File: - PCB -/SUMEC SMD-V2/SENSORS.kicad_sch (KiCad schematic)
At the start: 20 parts, among them U4 QRE1113, U5 QRE1113, U6 QRE1113

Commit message: cleanup
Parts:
- U4, U5, U6: footprint sumec_library:OnSemi_CASE100AQ - QRE1113 -> (none)
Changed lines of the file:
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@@
       (effects (font (size 1.27 1.27)) (justify left))
     )
-    (property "Footprint" "sumec_library:OnSemi_CASE100AQ - QRE1113" (at 218.44 92.71 0)
+    (property "Footprint" "" (at 218.44 92.71 0)
       (effects (font (size 1.27 1.27)) hide)
     )
@@
       (effects (font (size 1.27 1.27)) (justify left))
     )
-    (property "Footprint" "sumec_library:OnSemi_CASE100AQ - QRE1113" (at 182.88 92.71 0)
+    (property "Footprint" "" (at 182.88 92.71 0)
       (effects (font (size 1.27 1.27)) hide)
     )
@@
       (effects (font (size 1.27 1.27)) (justify left))
     )
-    (property "Footprint" "sumec_library:OnSemi_CASE100AQ - QRE1113" (at 200.66 92.71 0)
-      (effects (font (size 1.27 1.27)) hide)
-    )
+    (property "Footprint" "" (at 200.66 92.71 0)
+      (effects (font (size 1.27 1.27)) hide)
+    )

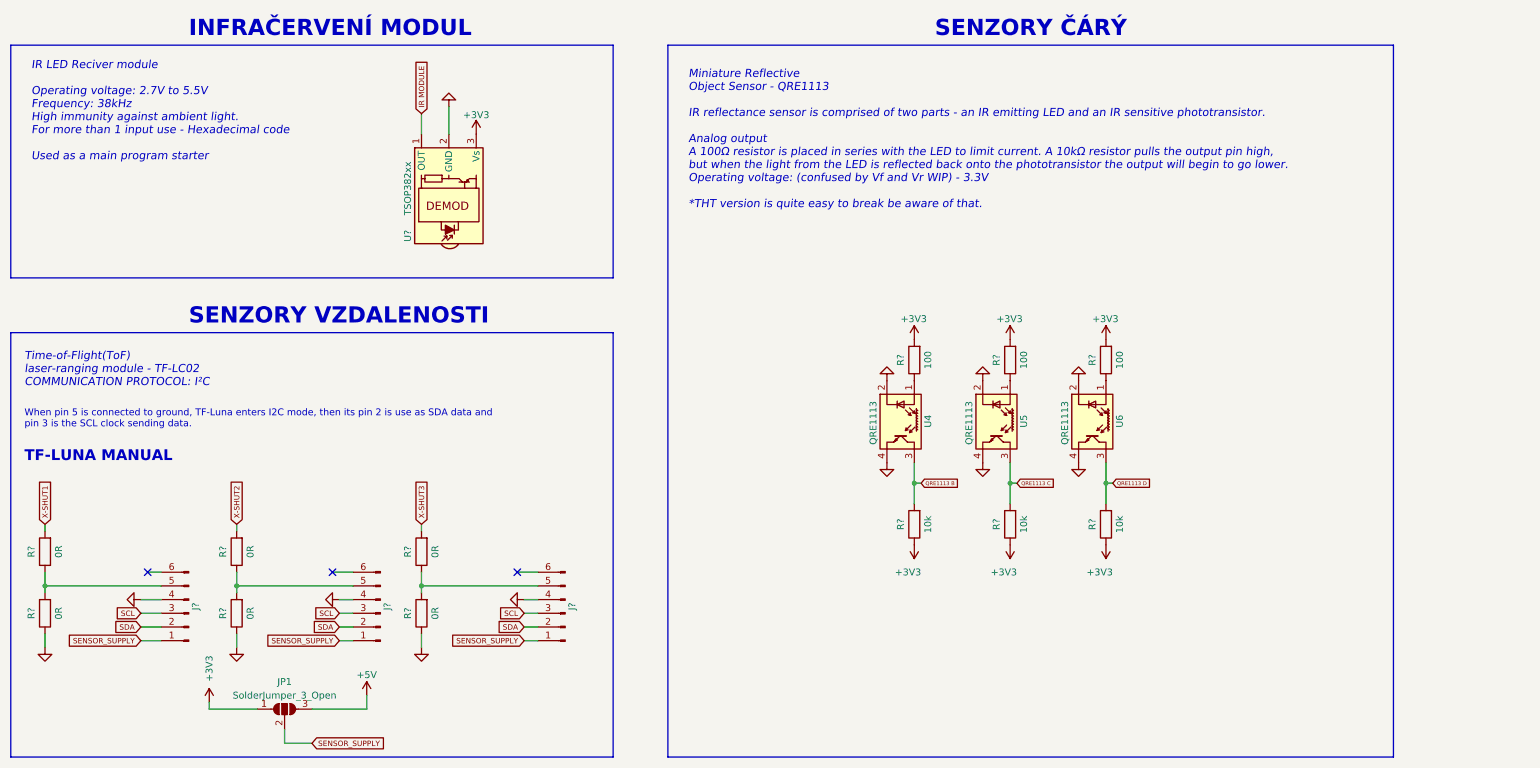
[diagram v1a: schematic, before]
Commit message: sumec SMD V2 schematic update
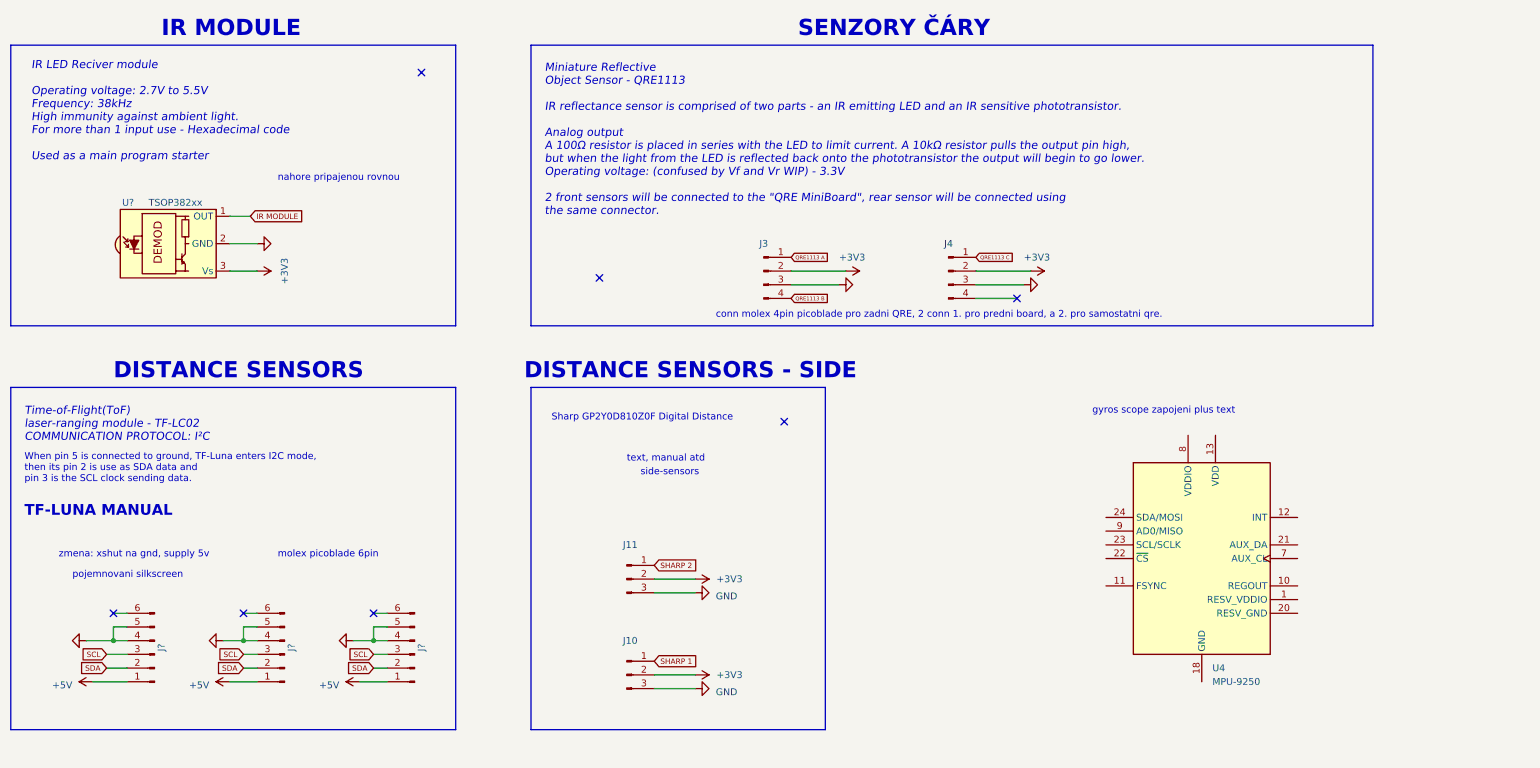
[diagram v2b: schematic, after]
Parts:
- removed J?: Conn_01x06_Pin, Connector_JST:JST_SH_BM06B-SRSS-TB_1x06-1MP_P1.00mm_Vertical, symbol Connector:Conn_01x06_Pin
- removed JP1: SolderJumper_3_Open, Jumper:SolderJumper-3_P2.0mm_Open_TrianglePad1.0x1.5mm, symbol Jumper:SolderJumper_3_Open
- removed R? (x3): 100, Resistor_SMD:R_1206_3216Metric, symbol Device:R
- removed R? (x6): 0R, Resistor_SMD:R_1206_3216Metric, symbol Device:R
- removed R? (x3): 10k, Resistor_SMD:R_1206_3216Metric, symbol Device:R
- removed U4, U5, U6: QRE1113, symbol Sensor_Proximity:QRE1113
- removed U?: TSOP382xx, Connector_PinSocket_2.54mm:PinSocket_1x03_P2.54mm_Vertical, symbol Interface_Optical:TSOP382xx
- added J10, J11: Conn_01x03_Pin, Connector_PinHeader_2.54mm:PinHeader_1x03_P2.54mm_Vertical, symbol Connector:Conn_01x03_Pin
- added J3, J4: Conn_01x04_Pin, Connector_Molex:Molex_PicoBlade_53398-0471_1x04-1MP_P1.25mm_Vertical, symbol Connector:Conn_01x04_Pin
- added J?: Conn_01x06_Pin, symbol Connector:Conn_01x06_Pin
- added U4: MPU-9250, Sensor_Motion:InvenSense_QFN-24_3x3mm_P0.4mm, symbol Sensor_Motion:MPU-9250
- added U?: TSOP382xx, Connector_PinSocket_2.54mm:PinSocket_1x03_P2.54mm_Vertical, symbol Interface_Optical:TSOP382xx
- J? (x2): footprint Connector_JST:JST_SH_BM06B-SRSS-TB_1x06-1MP_P1.00mm_Vertical -> (none)
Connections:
- net SENSOR_SUPPLY is gone; now on net +5V: J?.1 (Pin_1), J?.1 (Pin_1)
- net +3V3: now also J10.2 (Pin_2), J11.2 (Pin_2), J3.2 (Pin_2), J4.2 (Pin_2), U?.3 (Vs)
- net +5V: now also J?.1 (Pin_1)
- net GND: now also J?.5 (Pin_5), J?.5 (Pin_5), J10.3 (Pin_3), J11.3 (Pin_3), J3.3 (Pin_3), J4.3 (Pin_3), J?.4 (Pin_4), J?.5 (Pin_5), U?.2 (GND)
- net IR MODULE: now also U?.1 (OUT)
- net QRE1113 B: now also J3.4 (Pin_4)
- net QRE1113 C: now also J4.1 (Pin_1)
- net SCL: now also J?.3 (Pin_3)
- net SDA: now also J?.2 (Pin_2)
- new net QRE1113 A: J3.1 (Pin_1)
- new net SHARP 1: J10.1 (Pin_1)
- new net SHARP 2: J11.1 (Pin_1)
- no-connect marks 3 -> 7
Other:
- note added: "DISTANCE SENSORS"
- note added: "DISTANCE SENSORS - SIDE"
- note added: "IR MODULE"
- note added: "SENZORY ČÁRY"
- note added: "Sharp GP2Y0D810Z0F Digital Distance"
- note added: "conn molex 4pin picoblade pro zadni QRE, 2 conn 1. pro predni board, a 2. pro samostatni qre."
- note added: "gyros scope zapojeni plus text"
- note added: "molex picoblade 6pin"
- note added: "nahore pripajenou rovnou"
- note added: "pojemnovani silkscreen"
- note added: "side-sensors"
- note added: "text, manual atd"
- note added: "zmena: xshut na gnd, supply 5v"
- note removed: "INFRAČERVENÍ MODUL"
- note removed: "SENZORY VZDALENOSTI"
- note removed: "SENZORY ČÁRÝ"
- moved on the sheet: J?
